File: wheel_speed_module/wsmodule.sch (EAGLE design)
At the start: 19 parts, among them T1 BC849, U1 LTC2875XS

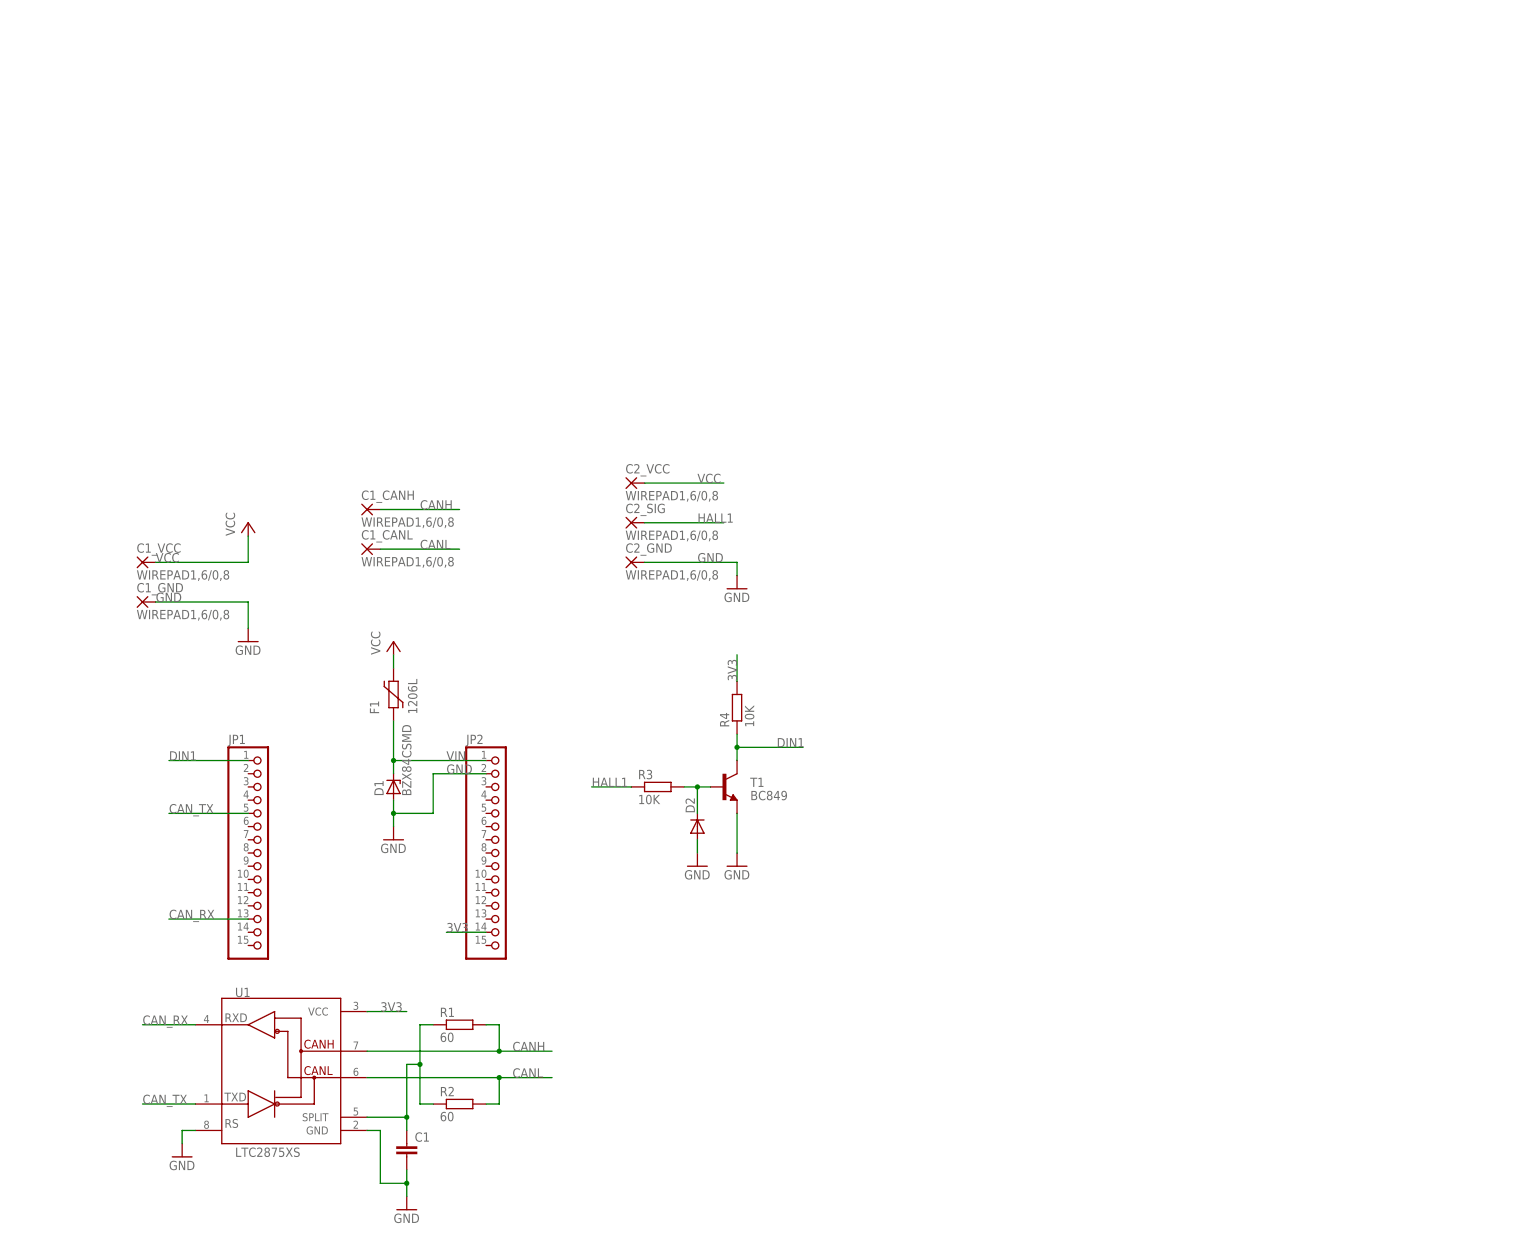
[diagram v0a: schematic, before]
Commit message: Version 1.1
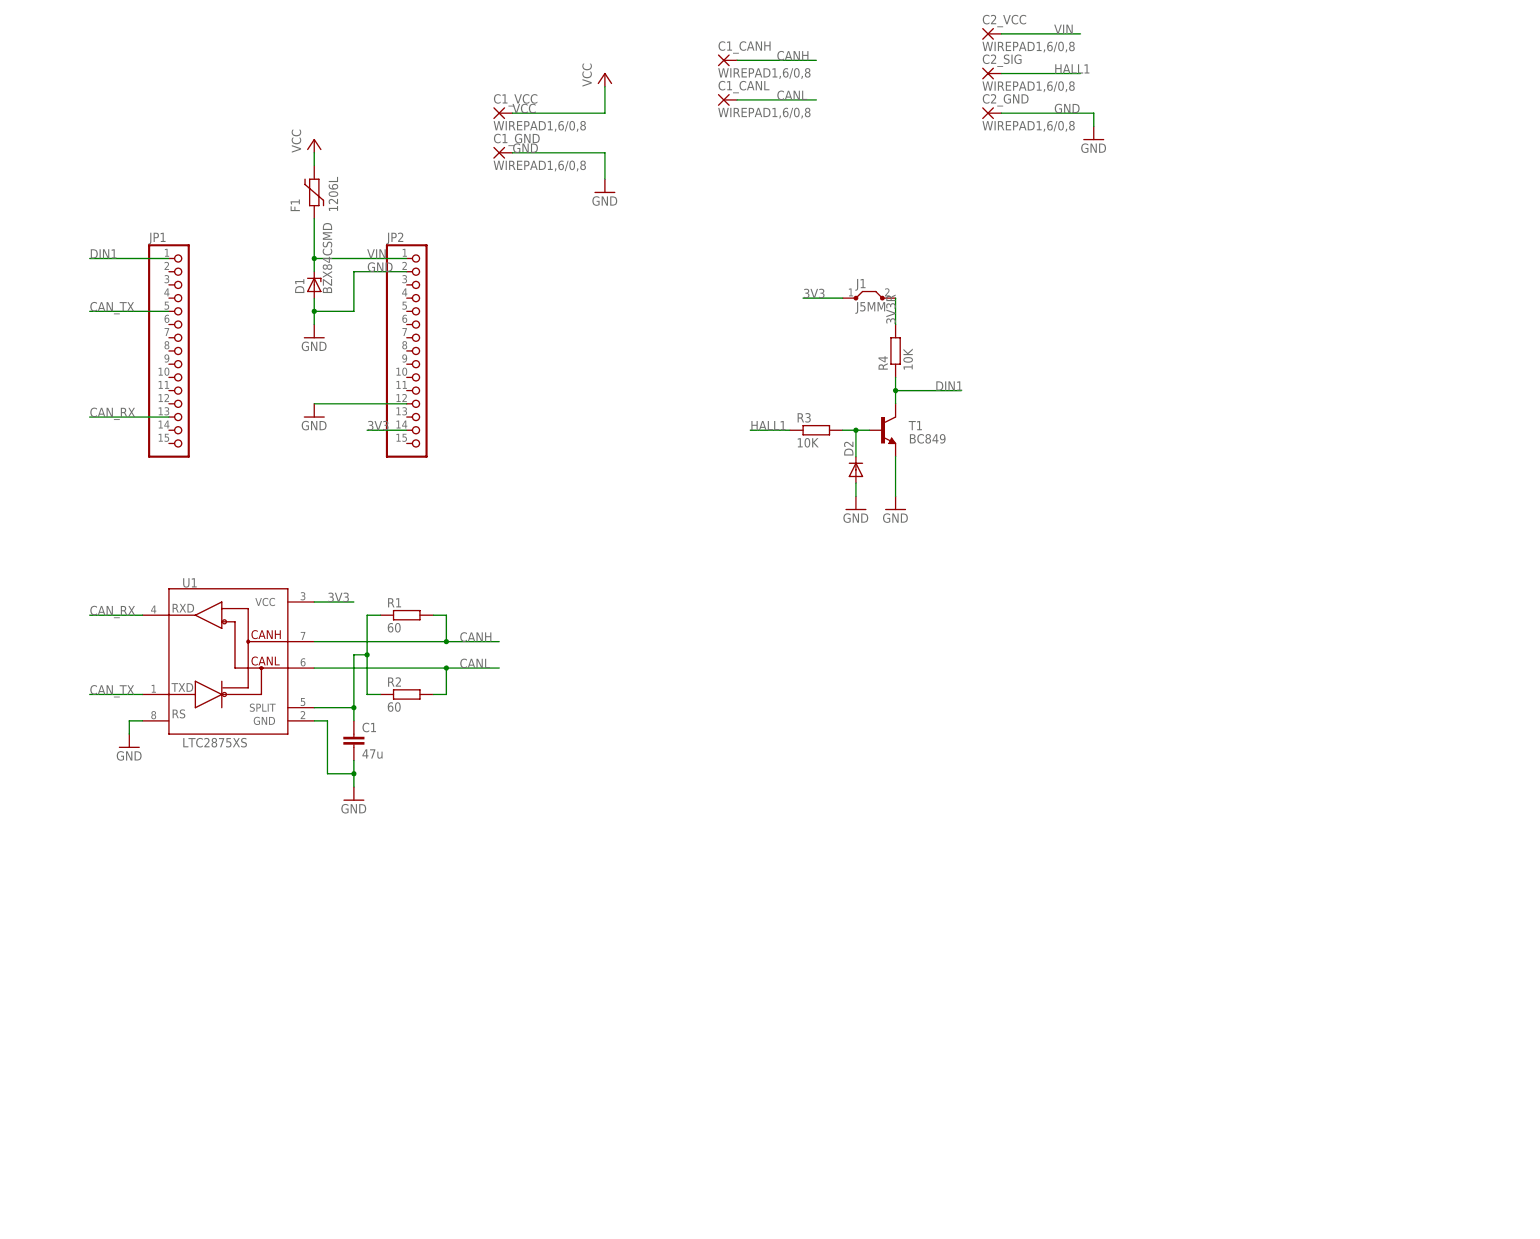
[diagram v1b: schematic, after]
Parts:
- added J1: J5MM, jumper:J5MM
- C1: value (none) -> 47u; device eagle-ltspice:C -> eagle-ltspice:CC1210
- R1, R2, R3, R4: device eagle-ltspice:R -> eagle-ltspice:RR1206
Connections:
- new net 3V3R: J1.2, R4.2
- net 3V3: now also J1.1; no longer R4.2
- net GND: now also JP2.12
- net VCC: no longer C2_VCC.P
- net VIN: now also C2_VCC.P
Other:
- moved on the sheet: C1, C1_CANH, C1_CANL, C1_GND, C1_VCC, C2_GND, C2_SIG, C2_VCC, D1, D2, F1, JP1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

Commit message: Version 1.2
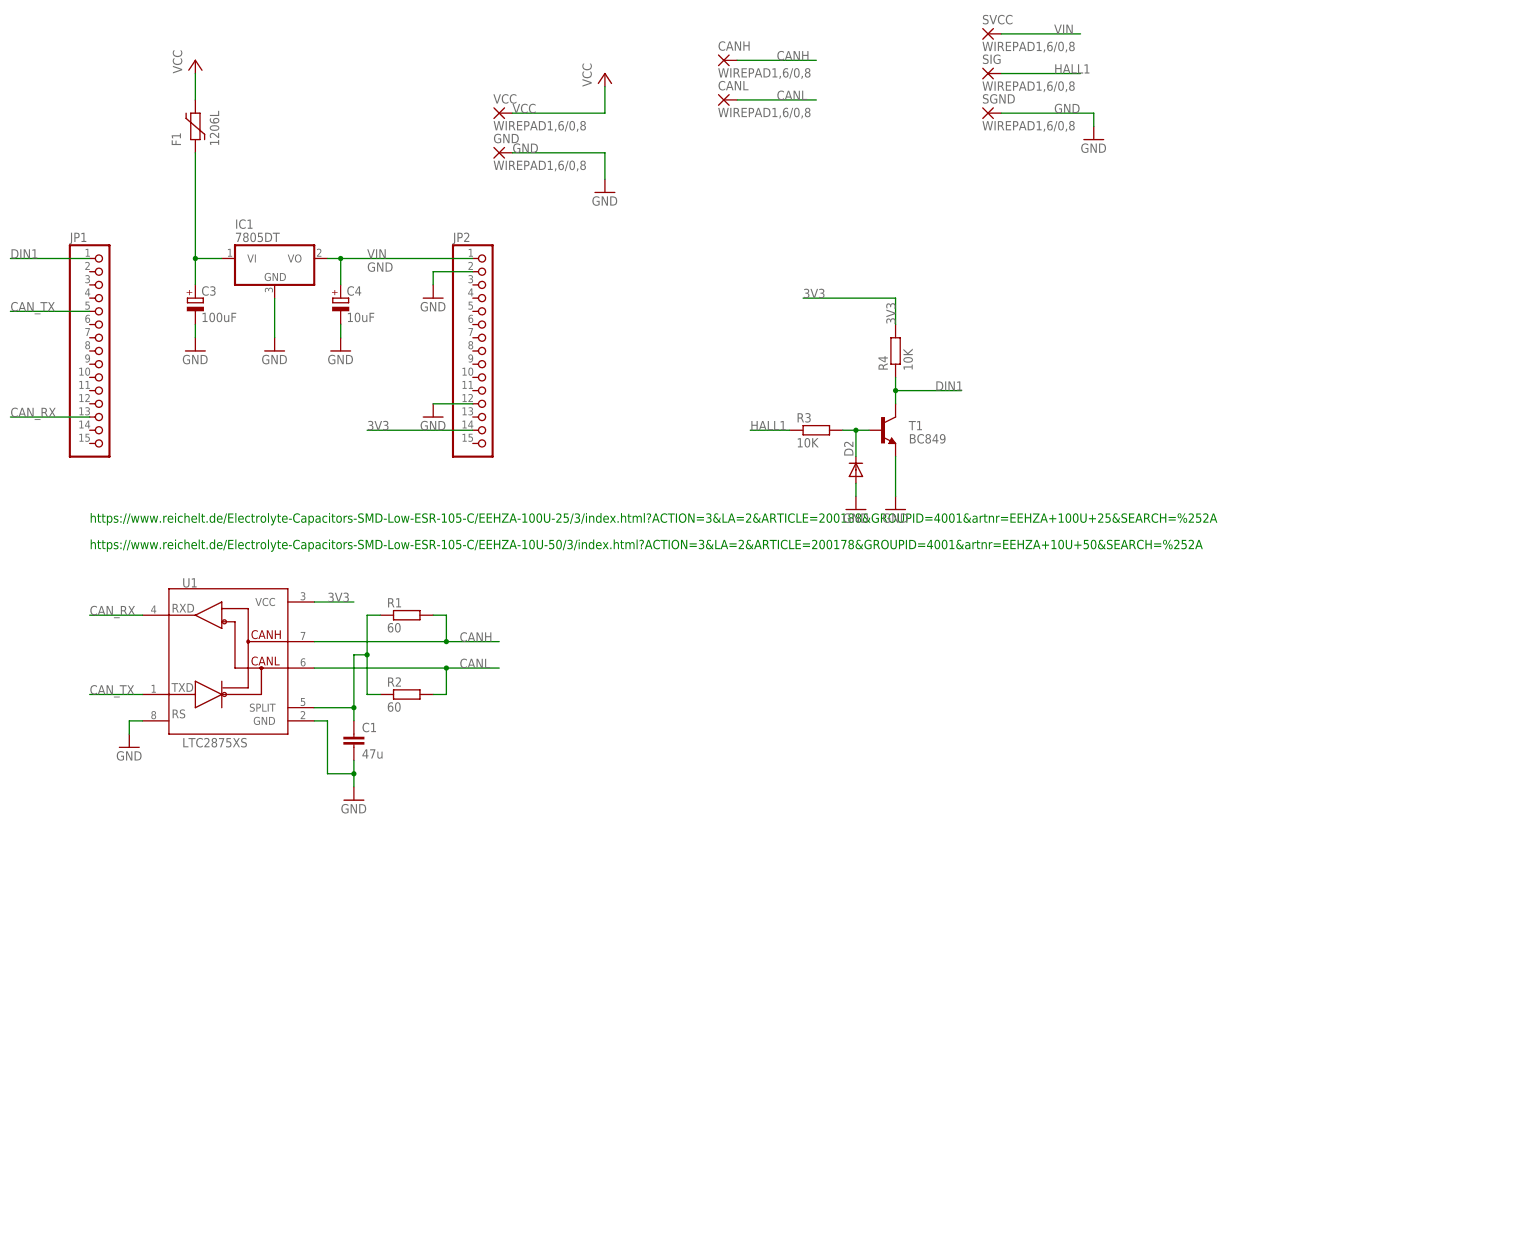
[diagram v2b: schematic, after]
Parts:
- removed D1: BZX84CSMD, diode:BZX84CSMD
- removed J1: J5MM, jumper:J5MM
- added C3: 100uF, rcl:CPOL-EUD
- added C4: 10uF, rcl:CPOL-EUC
- added IC1: 7805DT, linear:7805DT
- renumbered C1_CANH to CANH, C1_CANL to CANL, C1_GND to GND, C1_VCC to VCC, C2_GND to SGND, C2_SIG to SIG, C2_VCC to SVCC
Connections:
- removed net 3V3R: J1.2, R4.2
- new net N$2: C4.+, IC1.VO, JP2.1
- net 3V3: now also R4.2; no longer J1.1
- net GND: now also C3.-, C4.-, IC1.GND; no longer D1.A
- net VIN: now also C3.+, IC1.VI; no longer D1.C, JP2.1
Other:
- note added: "https://www.reichelt.de/Electrolyte-Capacitors-SMD-Low-ESR-105-C/EEHZA-100U-25/3/index.html?ACTION=3&LA=2&ARTICLE=200188&GROUPID=4001&artnr=EEHZA+100U+25&SEARCH=%252A"
- note added: "https://www.reichelt.de/Electrolyte-Capacitors-SMD-Low-ESR-105-C/EEHZA-10U-50/3/index.html?ACTION=3&LA=2&ARTICLE=200178&GROUPID=4001&artnr=EEHZA+10U+50&SEARCH=%252A"
- moved on the sheet: F1, JP1, JP2
